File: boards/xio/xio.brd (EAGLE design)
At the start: 170 x 170 mm, 390 parts, among them U2 LAN8742A-CZ, Y1 NX3225SA-12.000MHZ-STD-CSR-1, Y2 NX3225SA-12.000MHZ-STD-CSR-1, Y3 NX3225SA-25.000MHZ-STD-CSR-1

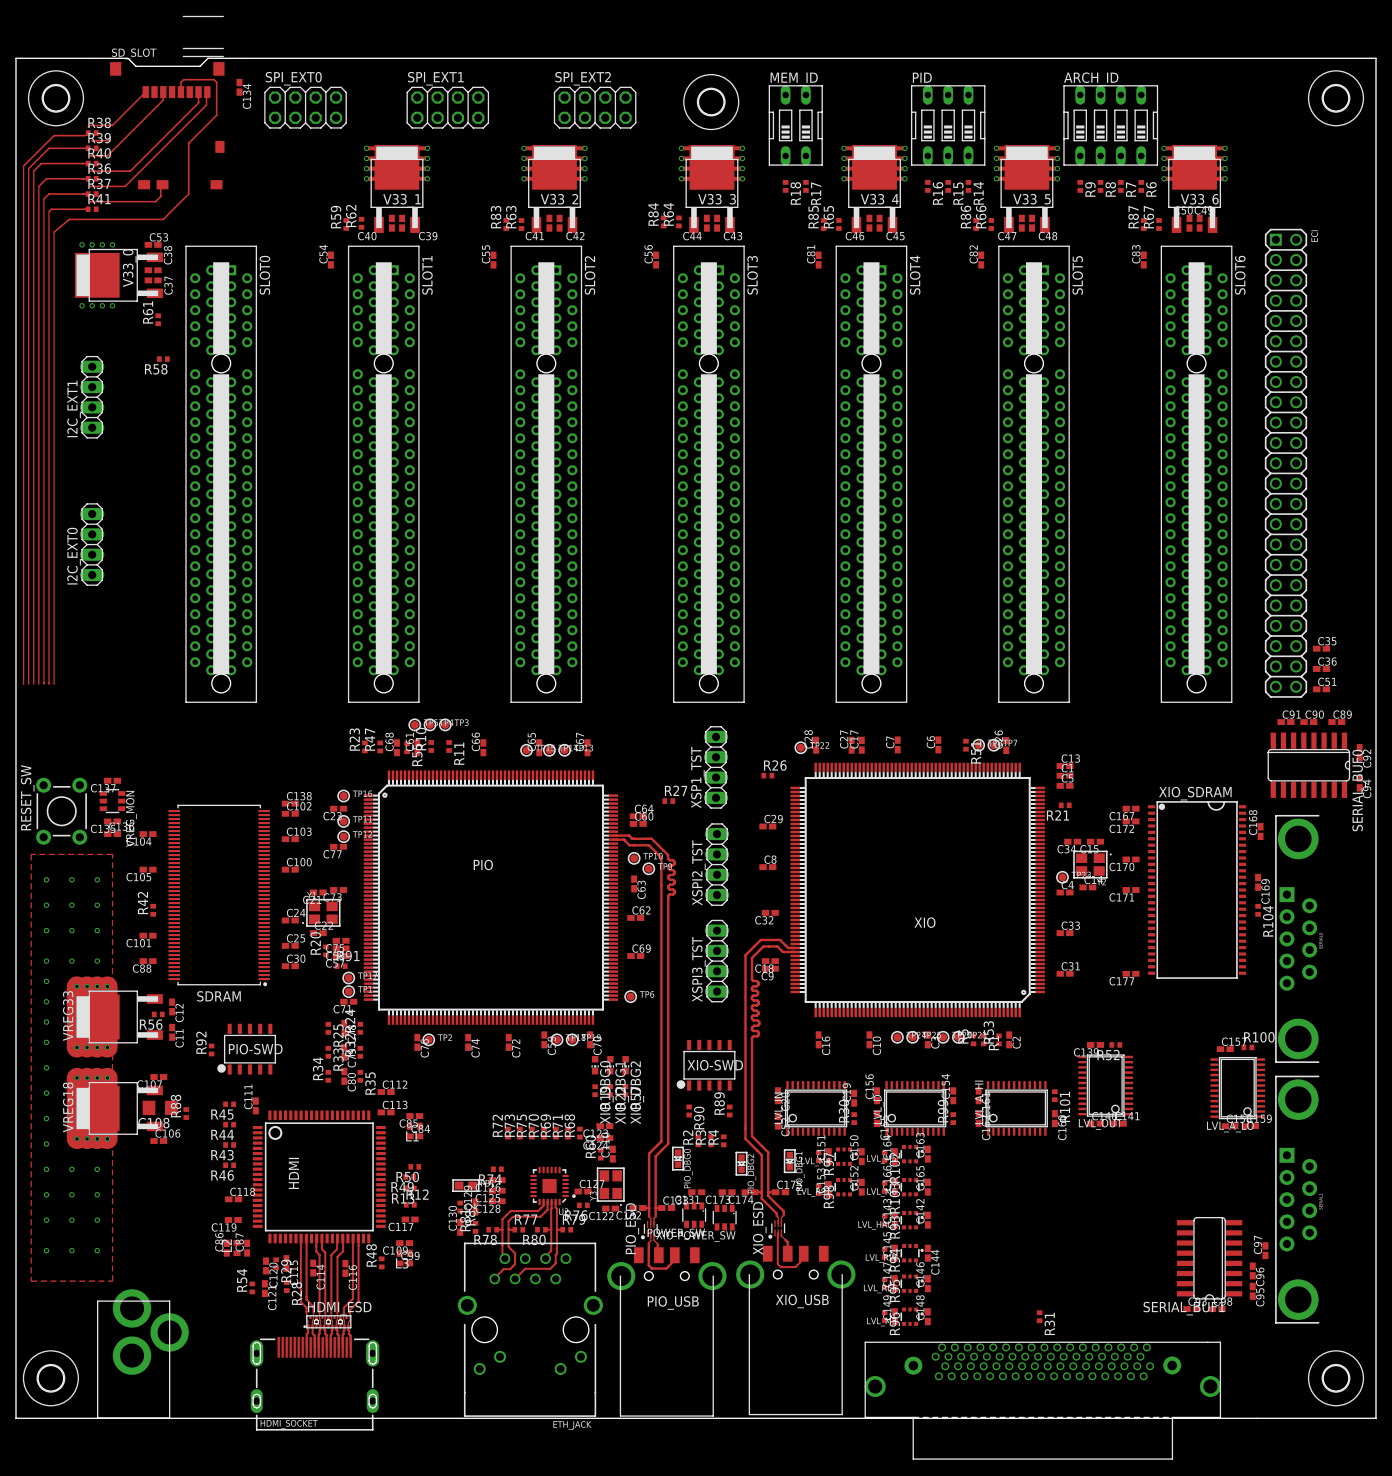
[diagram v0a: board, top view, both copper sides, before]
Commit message: Latest board layout
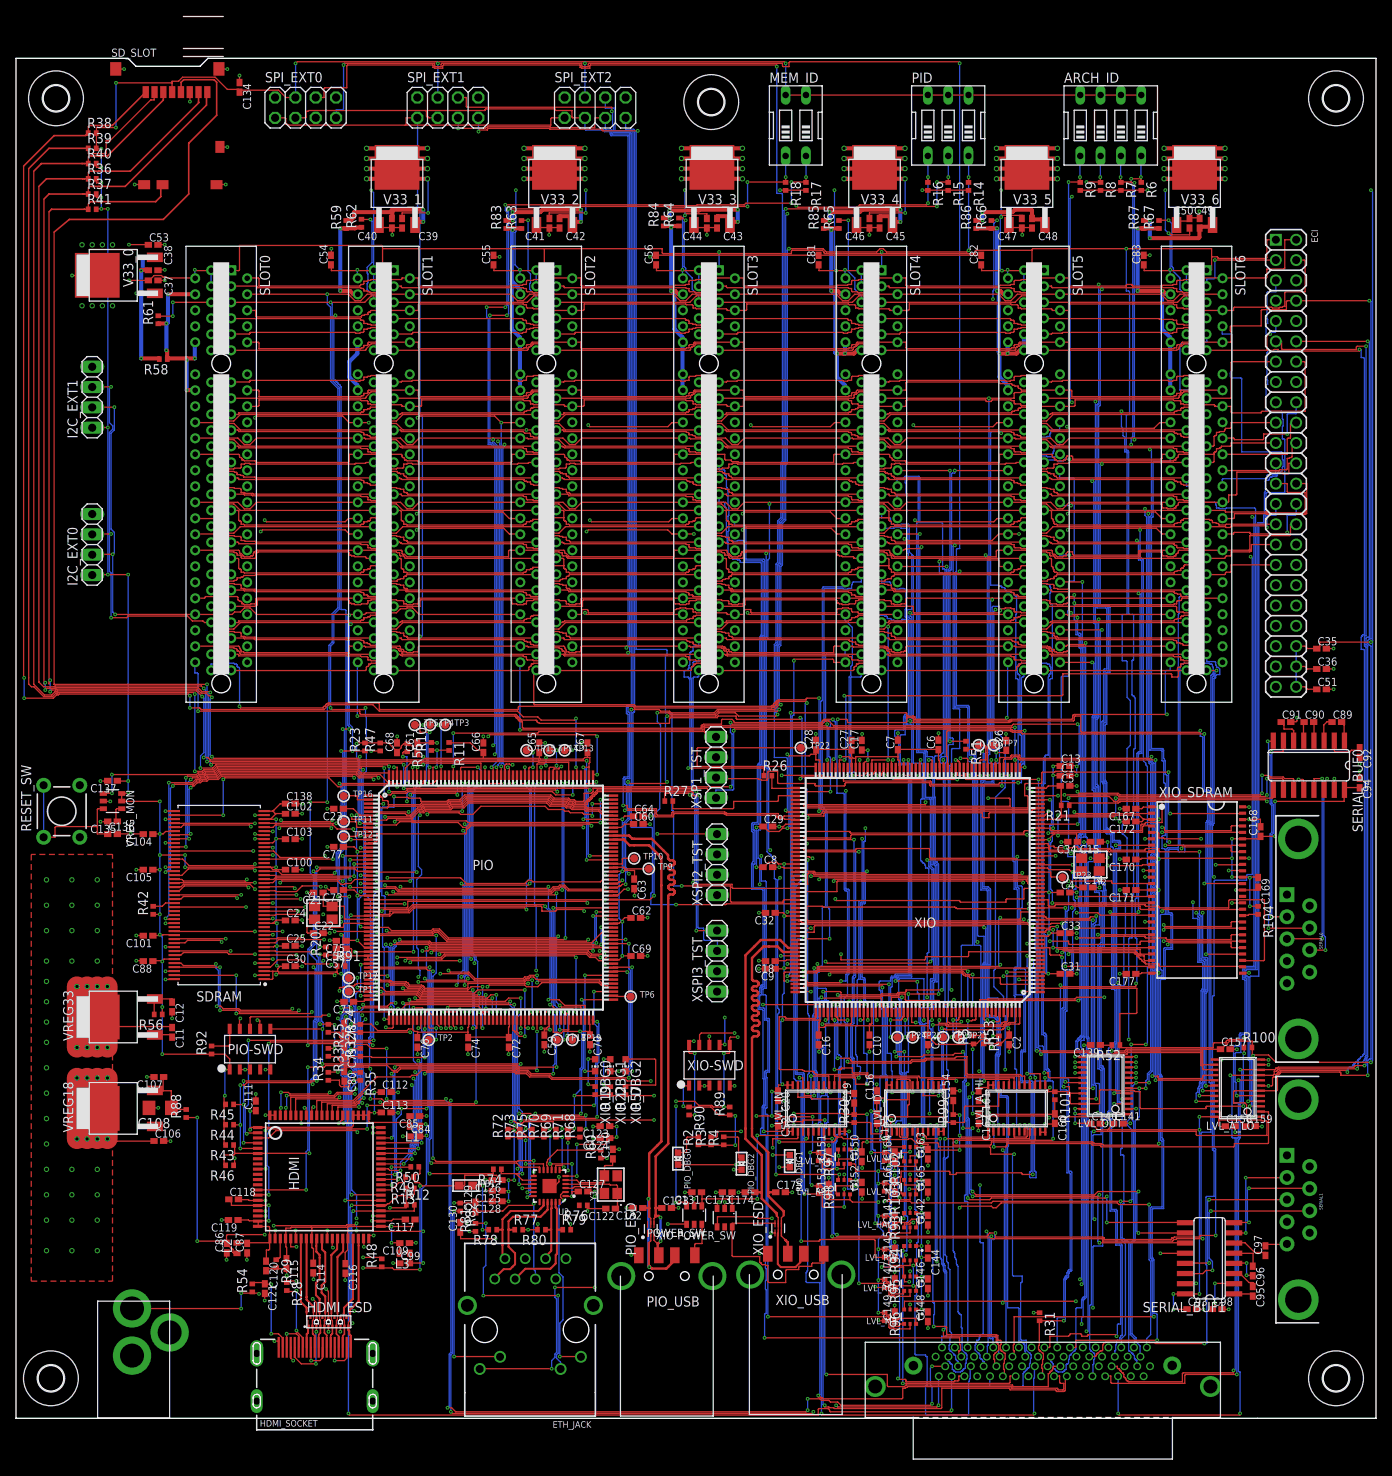
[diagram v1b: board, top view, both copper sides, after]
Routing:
- net +3V3: track 0.00 -> 1208.2 mm, vias 0 -> 144
- net +5V: track 165.5 -> 732.9 mm, vias 104 -> 161
- net GND: track 0.00 -> 374.2 mm, vias 0 -> 264
- net VHDCI_AUDIO_SIO: track 0.00 -> 368.6 mm, vias 0 -> 4
- net VHDCI_AUDIO_L: track 0.00 -> 356.3 mm, vias 0 -> 12
- net VHDCI_AUDIO_R: track 0.00 -> 350.3 mm, vias 0 -> 10
- net VHDCI_A3: track 0.00 -> 333.5 mm, vias 0 -> 3
- net VHDCI_RD4: track 0.00 -> 323.5 mm, vias 0 -> 4
- net VHDCI_A7: track 0.00 -> 322.0 mm, vias 0 -> 5
- net VHDCI_RD5: track 0.00 -> 320.2 mm, vias 0 -> 5
- net VHDCI_A6: track 0.00 -> 317.0 mm, vias 0 -> 4
- net VHDCI_D1XX: track 0.00 -> 314.5 mm, vias 0 -> 5
- net VHDCI_CCTL: track 0.00 -> 313.3 mm, vias 0 -> 4
- net !VHDCI_EXSEL!: track 0.00 -> 307.7 mm, vias 0 -> 5
- net VHDCI_CLK: track 0.00 -> 306.9 mm, vias 0 -> 3
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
